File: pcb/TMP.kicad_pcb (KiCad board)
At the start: 2 copper layers, 54.1 x 30.5 mm, 37 parts, among them J1 Conn_01x02_Pin, J2 Conn_01x02_Pin, J3 Conn_01x02_Pin, J4 Conn_01x03_Socket, U1 LM358

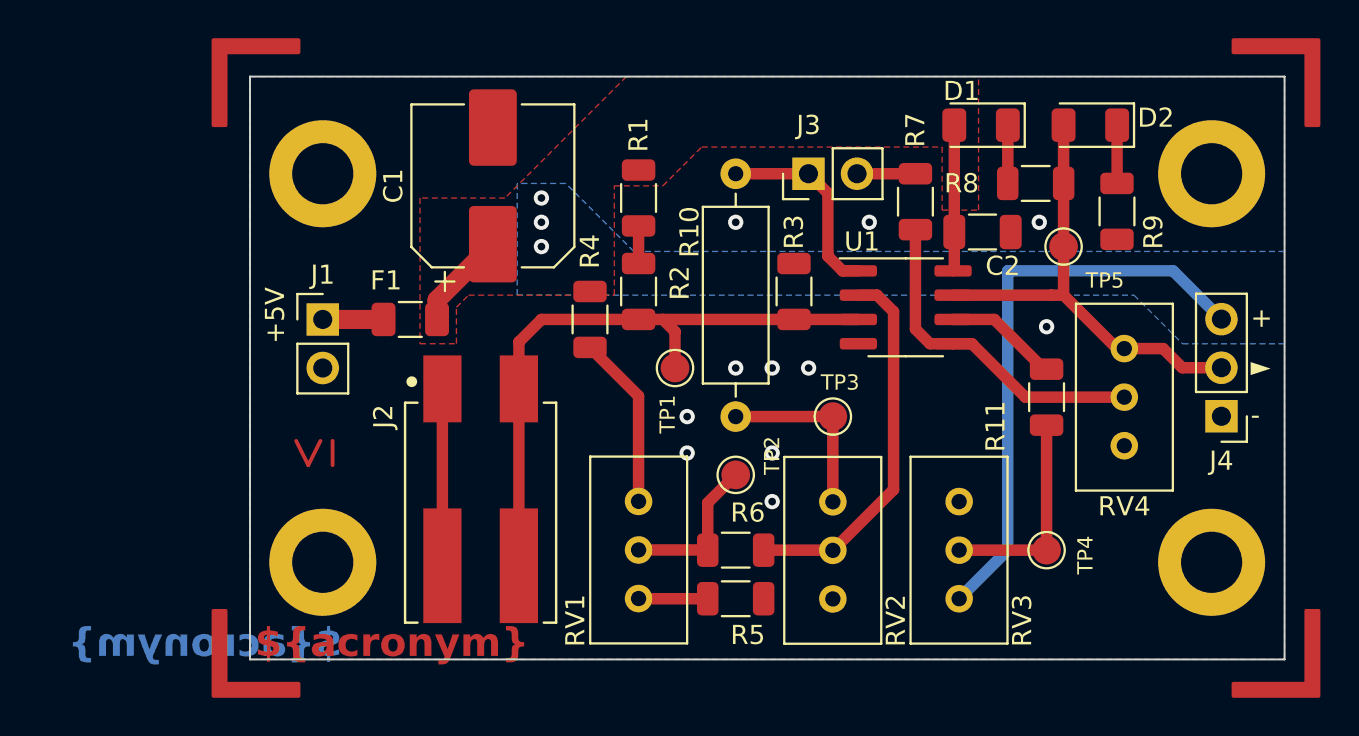
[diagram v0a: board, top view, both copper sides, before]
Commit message: Update to KiCAD 9
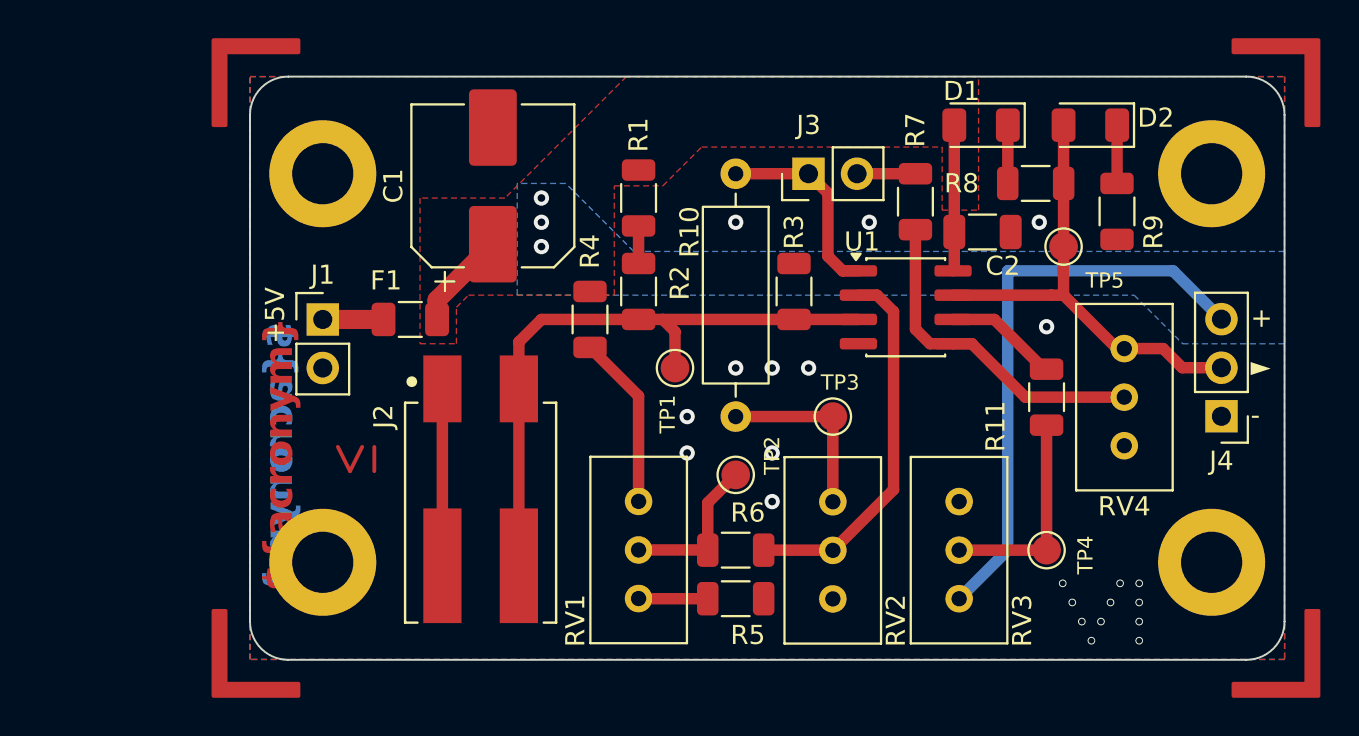
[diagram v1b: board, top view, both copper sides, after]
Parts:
- added FID4: QR, Images:QR_0x007e, B.Cu at (157.5, 87.3)
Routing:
- net GND: vias 11 -> 22
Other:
- outline, holes or cut-outs redrawn

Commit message: Rename fiducial to bin
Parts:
- FID2: value Waste -> BIN
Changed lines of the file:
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@@
 			)
 		)
-		(property "Value" "Waste"
+		(property "Value" "BIN"
 			(at 0.75 0 0)
 			(layer "B.Fab")
